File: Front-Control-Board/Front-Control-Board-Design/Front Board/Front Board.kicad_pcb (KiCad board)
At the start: 2 copper layers, 85.2 x 70.7 mm, 27 parts, among them J1 Conn_01x14, J2 Conn_01x14, J3 Conn_01x08, Q1 2N7002, U1 MAX33054EASA+T, U2 TS2940CP33 ROG, U3 ESP32-DevKitC

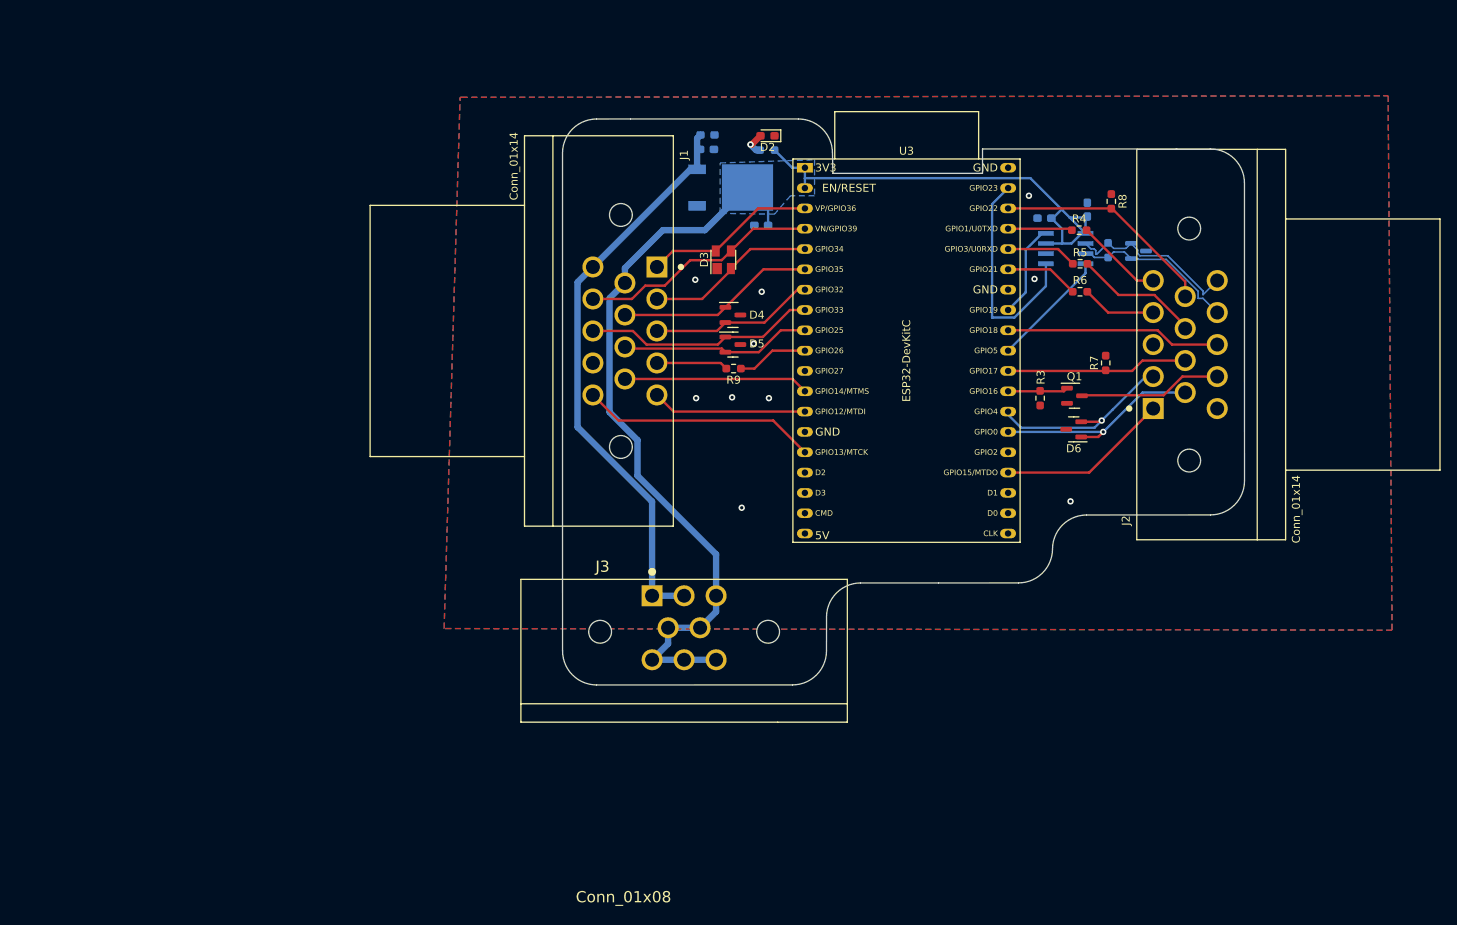
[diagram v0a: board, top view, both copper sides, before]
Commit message: updates
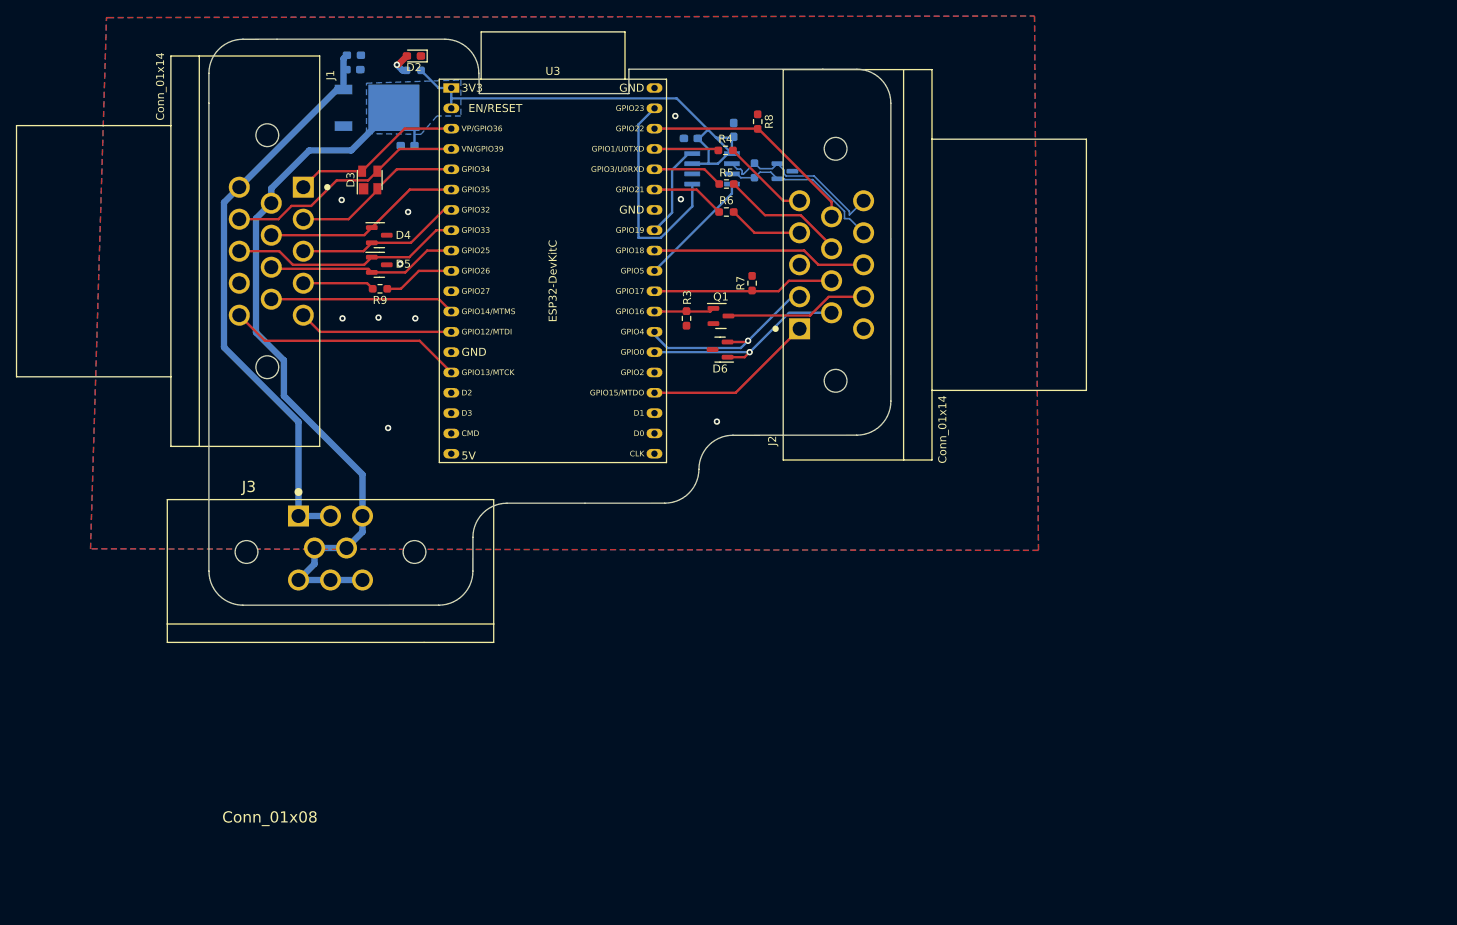
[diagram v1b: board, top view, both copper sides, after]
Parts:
- moved C2 45.3 mm to (132.1, 75.3)
- moved C4 45.3 mm to (167.5, 74.4)
- moved D4 45.3 mm to (128.6, 86.5)
- moved D5 45.3 mm to (128.6, 90.2)
- moved D6 45.3 mm to (171.2, 100.8)
- moved J1 45.3 mm to (115.1, 88.5)
- moved J2 45.3 mm to (185.1, 90.2)
- moved R4 45.3 mm to (171.9, 75.9)
- moved R7 45.3 mm to (175.2, 92.5)
- moved U1 45.3 mm to (170.2, 78.2)
- moved U2 45.3 mm to (128.3, 70.6)
- moved U3 45.3 mm to (137.6, 68.1)
- moved C1 45.3 mm to (125.4, 65.8)
- moved D7 45.3 mm to (125.4, 64.0)
- moved C3 45.3 mm to (172.9, 73.4)
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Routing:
- net /CAN_SCK: track 26.9 -> 0.00 mm
- net unconnected-(J2-Pad12): track 0.00 -> 26.9 mm
